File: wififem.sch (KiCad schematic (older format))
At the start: 38 parts, among them J1 Conn_Coaxial, J2 Conn_Coaxial, J3 Conn_Coaxial, J4 Conn_Coaxial, U1 MCP6566, U2 74HCT04, U3 SE2611T, U4 AP1117-15

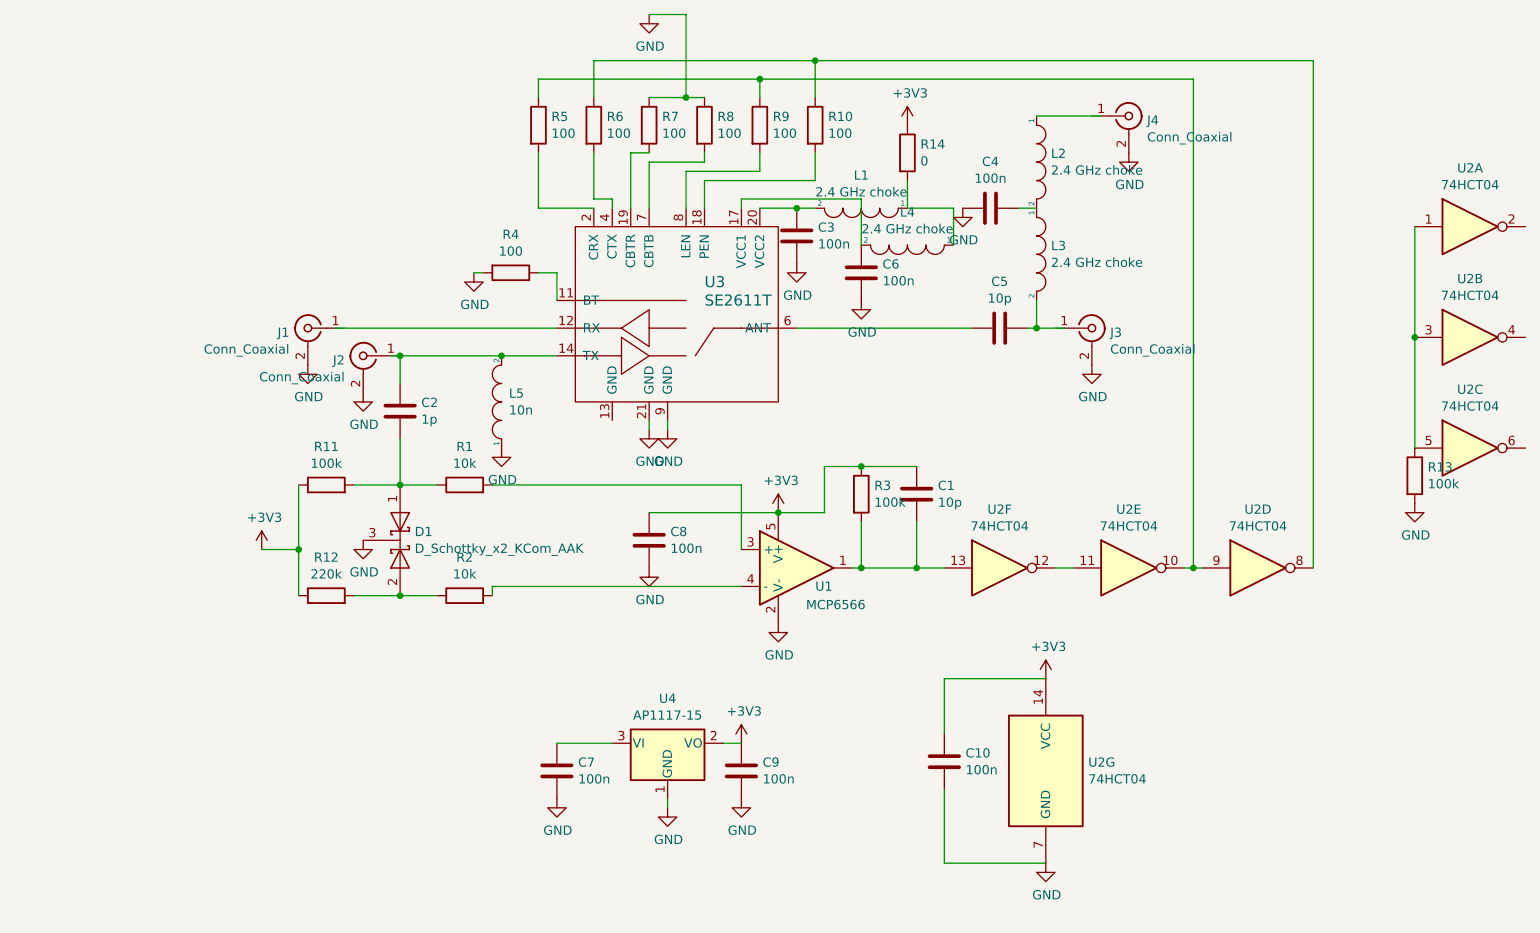
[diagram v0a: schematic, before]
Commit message: Everything in layout, DRC passes
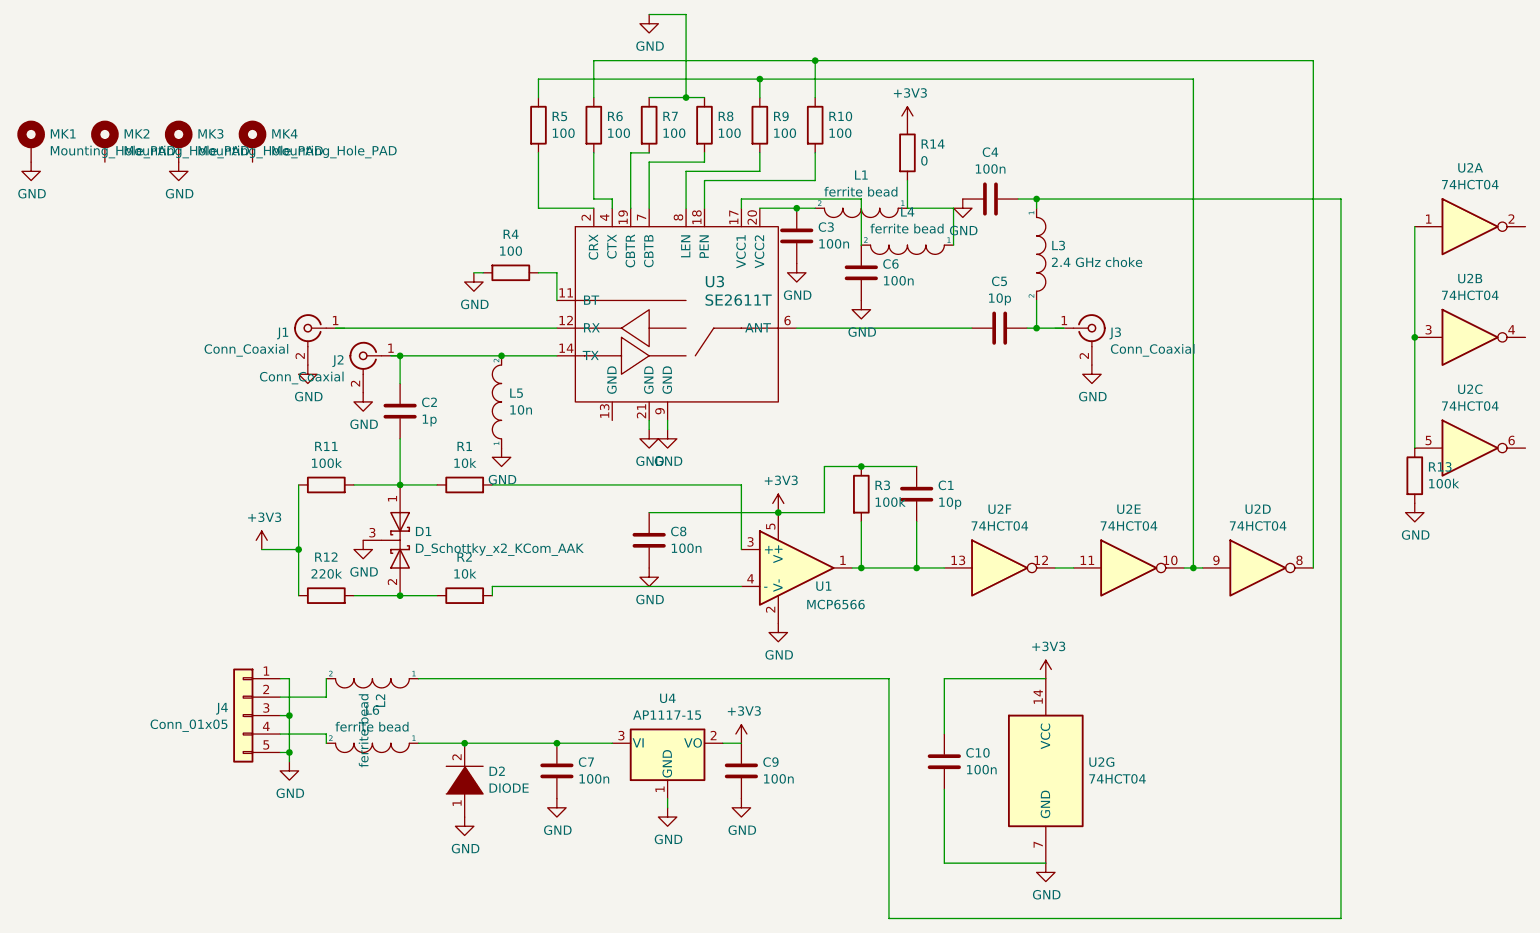
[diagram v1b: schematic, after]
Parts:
- removed J4: Conn_Coaxial, Connectors:SMA_THT_Jack_Straight, symbol Connector:Conn_Coaxial
- added D2: DIODE, Resistors_SMD:R_0805_HandSoldering, symbol pspice:DIODE
- added J4: Conn_01x05, Socket_Strips:Socket_Strip_Straight_1x05_Pitch2.54mm, symbol Connector:Conn_01x05
- added L6: ferrite bead, Inductors_SMD:L_0805_HandSoldering, symbol pspice:INDUCTOR
- added MK1, MK2, MK3, MK4: Mounting_Hole_PAD, Mounting_Holes:MountingHole_3.2mm_M3_Pad, symbol Mechanical:Mounting_Hole_PAD
- L1, L2, L4: value 2.4 GHz choke -> ferrite bead
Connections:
- wire segments 72 -> 84
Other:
- moved on the sheet: C4, L2
